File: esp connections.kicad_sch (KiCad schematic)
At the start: 3 parts, among them U1 ESP-12F, U2 STM8S003F3P

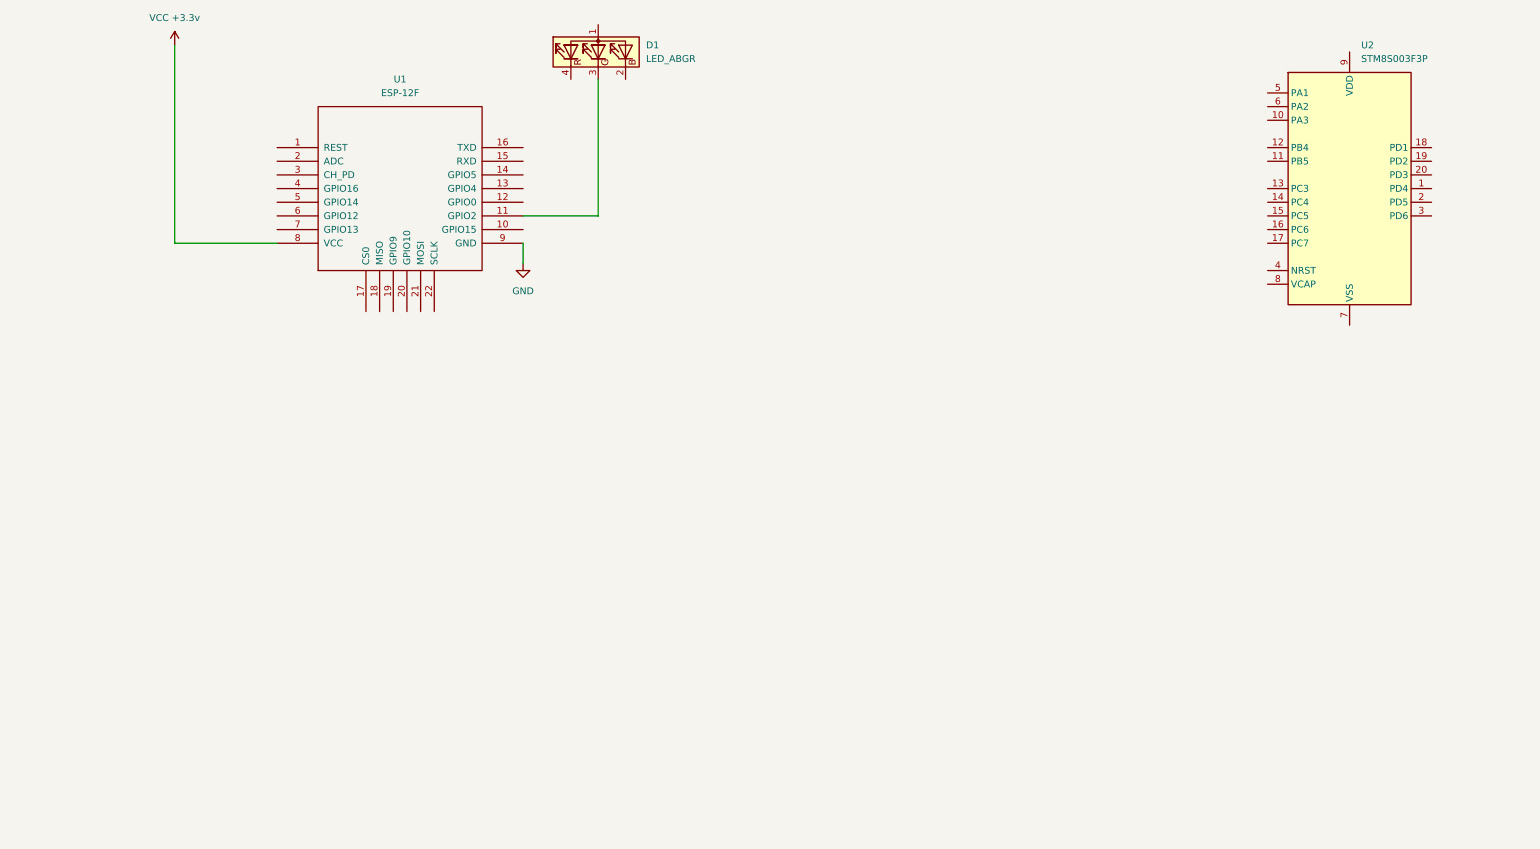
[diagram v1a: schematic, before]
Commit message: thursday 15th
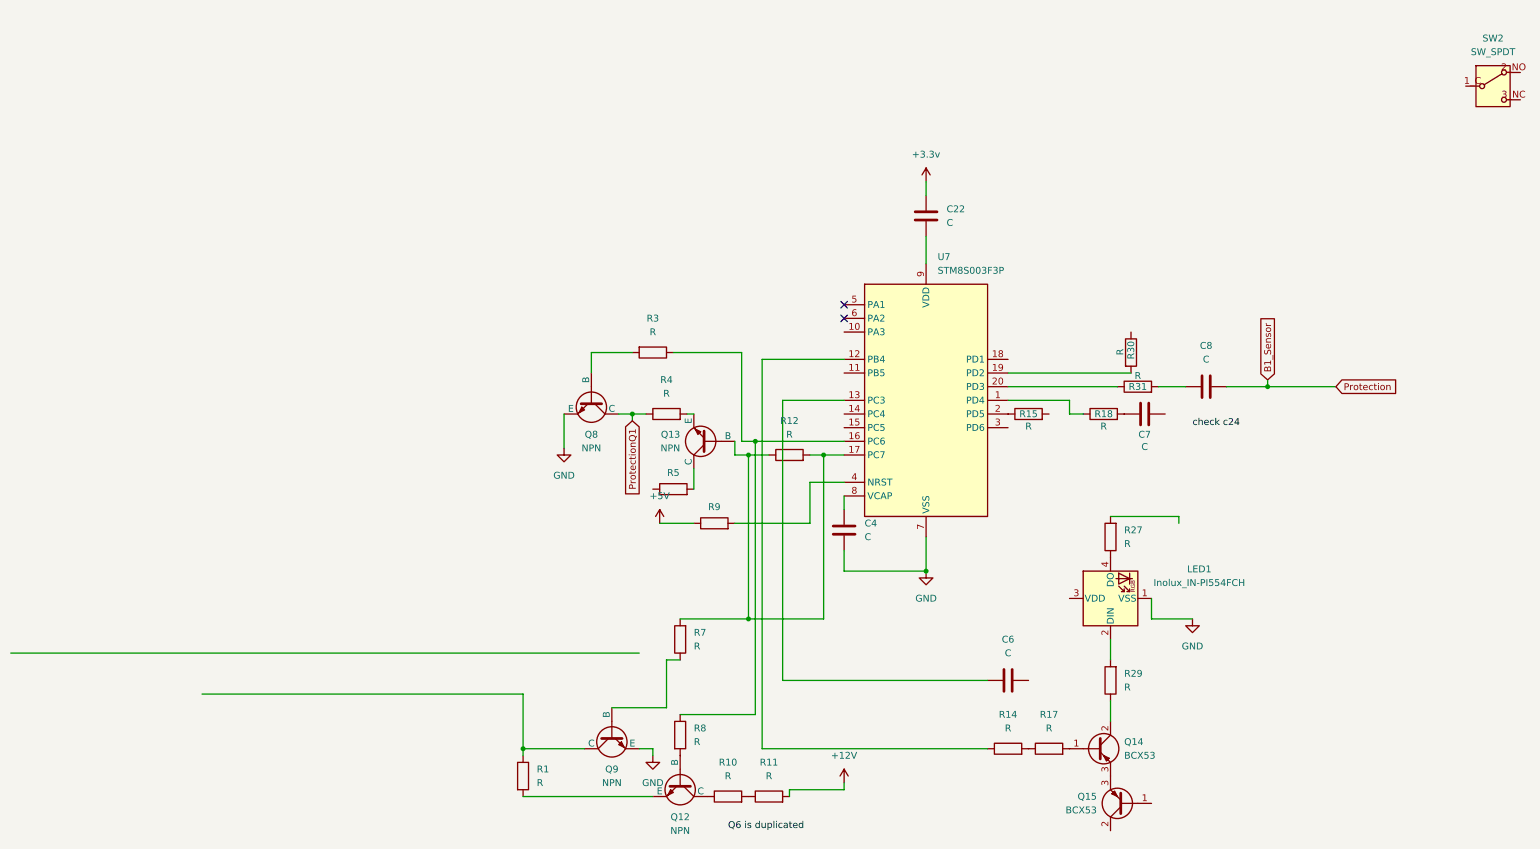
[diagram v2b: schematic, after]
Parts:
- removed D1: LED_ABGR, symbol Device:LED_ABGR
- removed U1: ESP-12F, symbol ESP8266:ESP-12F
- removed U2: STM8S003F3P, Package_SO:TSSOP-20_4.4x6.5mm_P0.65mm, symbol MCU_ST_STM8:STM8S003F3P
- added C22, C4, C6, C7, C8: C, symbol Device:C
- added LED1: Inolux_IN-PI554FCH, LED_SMD:LED_Inolux_IN-PI554FCH_PLCC4_5.0x5.0mm_P3.2mm, symbol LED:Inolux_IN-PI554FCH
- added Q12, Q13, Q8, Q9: NPN, symbol Simulation_SPICE:NPN
- added Q14, Q15: BCX53, Package_TO_SOT_SMD:SOT-89-3, symbol Transistor_BJT:BCX53
- added R1, R10, R11, R12, R14, R15, R17, R18, R27, R29, R3, R30, R31, R4, R5, R7, R8, R9: R, symbol Device:R
- added SW2: SW_SPDT, symbol Switch:SW_SPDT
- added U7: STM8S003F3P, Package_SO:TSSOP-20_4.4x6.5mm_P0.65mm, symbol MCU_ST_STM8:STM8S003F3P
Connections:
- net GND: now also C4.2, LED1.1 (VSS), Q8.3 (E), Q9.3 (E), U7.7 (VSS)
- new net: C4.1, U7.8 (VCAP)
- new net: R18.1, U7.1 (PD4)
- new net: C7.2, R18.2
- new net: R30.2, U7.19 (PD2)
- new net: R10.2, R11.1
- new net: LED1.4 (DO), R27.1
- new net: R15.1, U7.2 (PD5)
- new net: R14.1, U7.12 (PB4)
- new net: R14.2, R17.1
- new net: C6.1, U7.13 (PC3)
- new net: R3.1, R8.1, U7.16 (PC6)
- new net: Q13.2 (B), R12.1, R12.2, R7.2, U7.17 (PC7)
- new net: R31.1, U7.20 (PD3)
- new net: R9.2, U7.4 (NRST)
- new net: C22.2, U7.9 (VDD)
- new net: Q8.2 (B), R3.2
- new net: Q13.1 (C), R5.2
- new net: Q12.1 (C), R10.1
- new net: Q12.2 (B), R8.2
- new net: Q12.3 (E), R1.2
- new net: Q14.1 (B), R17.2
- new net: Q14.2 (C), R29.1
- new net: Q14.3 (E), Q15.3 (E)
- new net: Q9.2 (B), R7.1
- new net: Q9.1 (C), R1.1
- new net: Q13.3 (E), R4.2
- new net: C8.1, R31.2
- new net: LED1.2 (DIN), R29.2
- new net +12V: R11.2
- new net +3.3v: C22.1
- new net +5V: R9.1
- new net B1_Sensor: C8.2
- new net ProtectionQ1: Q8.1 (C), R4.1
- no-connect marks 0 -> 2

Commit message: new
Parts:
- removed C22, C4, C6, C7, C8: C, symbol Device:C
- removed LED1: Inolux_IN-PI554FCH, LED_SMD:LED_Inolux_IN-PI554FCH_PLCC4_5.0x5.0mm_P3.2mm, symbol LED:Inolux_IN-PI554FCH
- removed Q12, Q13, Q8, Q9: NPN, symbol Simulation_SPICE:NPN
- removed Q14, Q15: BCX53, Package_TO_SOT_SMD:SOT-89-3, symbol Transistor_BJT:BCX53
- removed R1, R10, R11, R12, R14, R15, R17, R18, R27, R29, R3, R30, R31, R4, R5, R7, R8, R9: R, symbol Device:R
- removed SW2: SW_SPDT, symbol Switch:SW_SPDT
- removed U7: STM8S003F3P, Package_SO:TSSOP-20_4.4x6.5mm_P0.65mm, symbol MCU_ST_STM8:STM8S003F3P
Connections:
- no-connect marks 2 -> 0
